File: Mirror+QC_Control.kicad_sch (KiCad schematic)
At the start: 29 parts, among them J1 3220-10-0300-00, J2 Screw_Terminal_01x04, J3 Screw_Terminal_01x06, U1 LT1012, U10 LT1012, U11 LT1012, U2 LM4040DBZ-2.0, U3 LT1012, U4 LM4040DBZ-2.0, U5 LT1012, U6 LT1012, U7 Teensy4.0

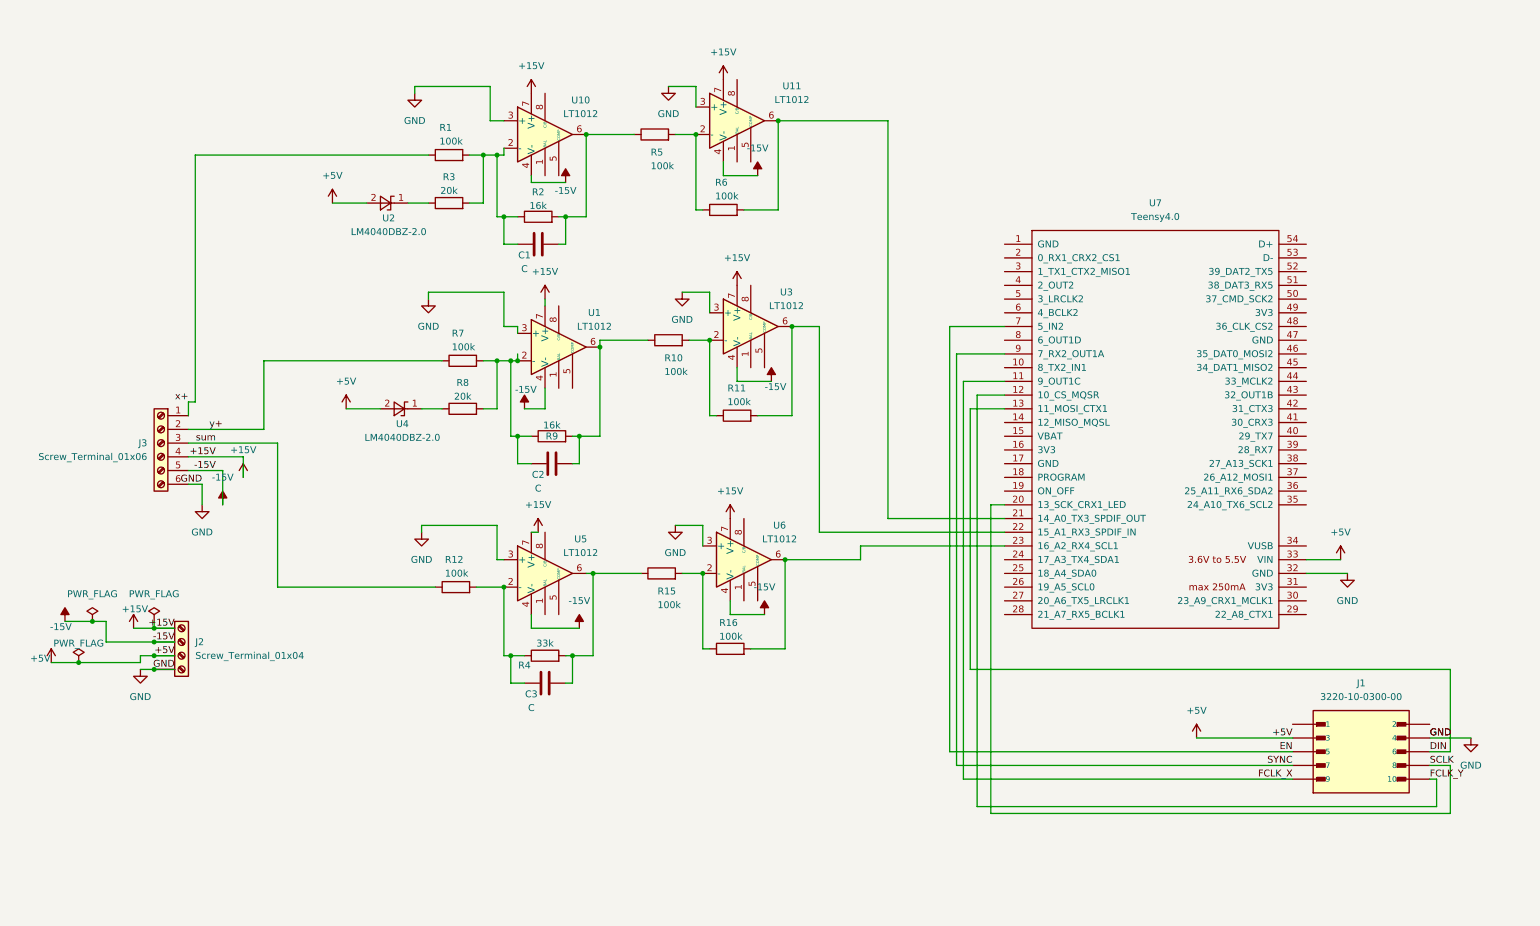
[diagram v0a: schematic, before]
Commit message: changes after DR1
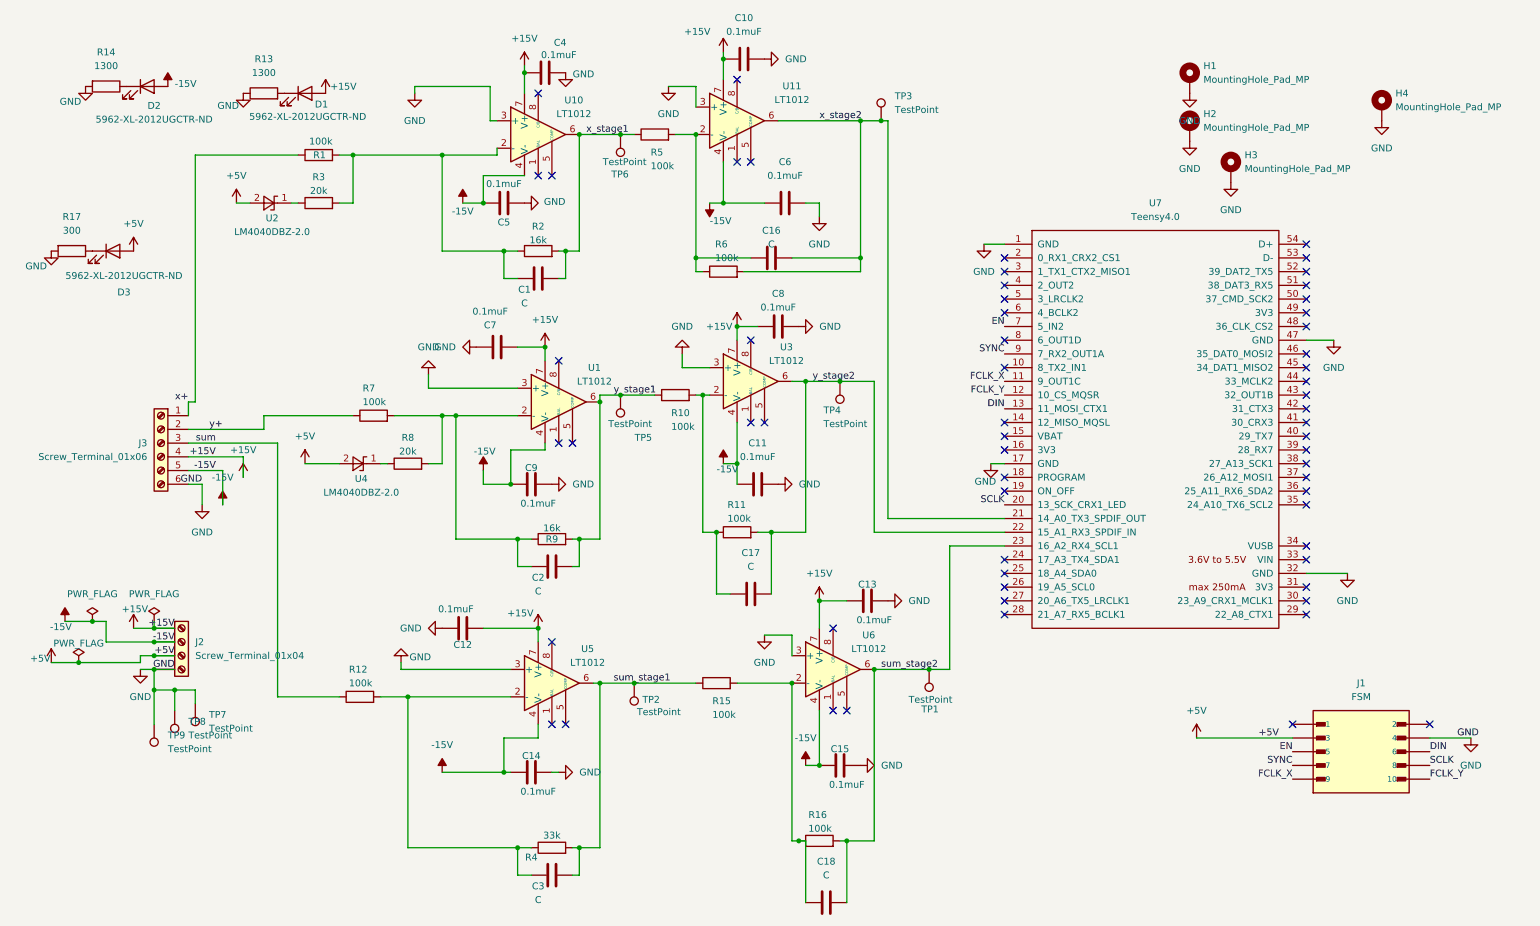
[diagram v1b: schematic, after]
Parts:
- added C10, C11, C12, C13, C14, C15, C4, C5, C6, C7, C8, C9: 0.1muF, Capacitor_SMD:C_0805_2012Metric, symbol Device:C
- added C16, C17, C18: C, Capacitor_SMD:C_0805_2012Metric, symbol Device:C
- added D1, D2, D3: 5962-XL-2012UGCTR-ND, LED_SMD:LED_0805_2012Metric, symbol Device:LED
- added H1, H2, H3, H4: MountingHole_Pad_MP, MountingHole:MountingHole_3.2mm_M3_DIN965_Pad_TopBottom, symbol Mechanical:MountingHole_Pad_MP
- added R13, R14: 1300, Resistor_SMD:R_0805_2012Metric, symbol Device:R
- added R17: 300, Resistor_SMD:R_0805_2012Metric, symbol Device:R
- added TP1, TP2, TP3, TP4, TP5, TP6, TP7, TP8, TP9: TestPoint, TestPoint:TestPoint_Pad_2.0x2.0mm, symbol Connector:TestPoint
- J1: value 3220-10-0300-00 -> FSM
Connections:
- net +15V: now also C10.2, C12.2, C13.2, C4.1, C7.2, C8.2, D1.2 (A)
- net +5V: now also D3.2 (A); no longer U7.33 (VIN)
- net -15V: now also C11.2, C14.2, C15.2, C5.1, C6.2, C9.2, D2.2 (A)
- net GND: now also U7.1 (GND), U7.17 (GND), U7.47 (GND), C10.1, C11.1, C12.1, C13.1, C14.1, C15.1, C4.2, C5.2, C6.1, C7.1, C8.1, C9.1, H1.MP, H2.MP, H3.MP, H4.MP, R13.1, R14.2, R17.2, TP7.1, TP8.1, TP9.1
- net sum_stage1: now reaches C3.2, R15.1, R4.2, U5.6
- net sum_stage1: now also TP2.1
- net at R15.2, R16.1, U6.2 (-): now also C18.1
- net y_stage1: now reaches C2.2, R10.1, R9.2, U1.6
- net y_stage1: now also TP5.1
- net at R10.2, R11.1, U3.2 (-): now also C17.1
- net x_stage1: now reaches C1.2, R2.2, R5.1, U10.6
- net x_stage1: now also TP6.1
- net at R5.2, R6.1, U11.2 (-): now also C16.1
- net y_stage2: now reaches R11.2, U3.6, U7.22 (15_A1_RX3_SPDIF_IN)
- net y_stage2: now also C17.2, TP4.1
- net sum_stage2: now reaches R16.2, U6.6, U7.23 (16_A2_RX4_SCL1)
- net sum_stage2: now also C18.2, TP1.1
- net x_stage2: now reaches R6.2, U11.6, U7.21 (14_A0_TX3_SPDIF_OUT)
- net x_stage2: now also C16.2, TP3.1
- new net: D1.1 (K), R13.2
- new net: D3.1 (K), R17.1
- new net: D2.1 (K), R14.1
- no-connect marks 0 -> 61
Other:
- title: (none) -> Teensy Control of QC and FSM
- moved on the sheet: C1, C2, C3, R1, R10, R11, R12, R15, R16, R2, R3, R4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
